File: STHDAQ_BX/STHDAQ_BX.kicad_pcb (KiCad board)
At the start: 2 copper layers, 36 x 56 mm, 52 parts, among them J1 532611071, P1 S2B-PH-SM4-TB, U1 ADS1256IDBR, U2 ADP151AUJZ-3.0-R7, U3 OPA350UA, U4 REF5025AIDR, U5 102010448, U6 LT1461AIS8-5-PBF, Y1 ABLS-8MHZ-K4T

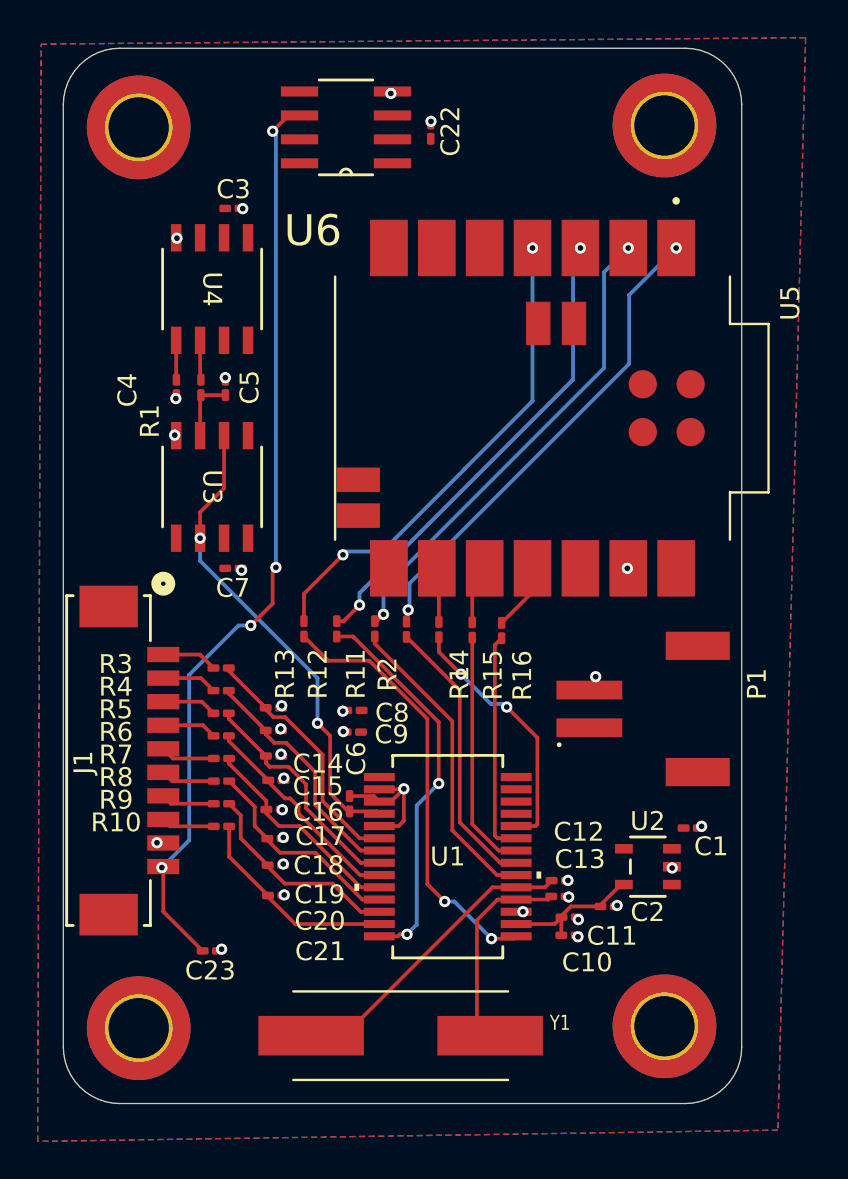
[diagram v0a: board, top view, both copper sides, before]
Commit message: Changes in BX
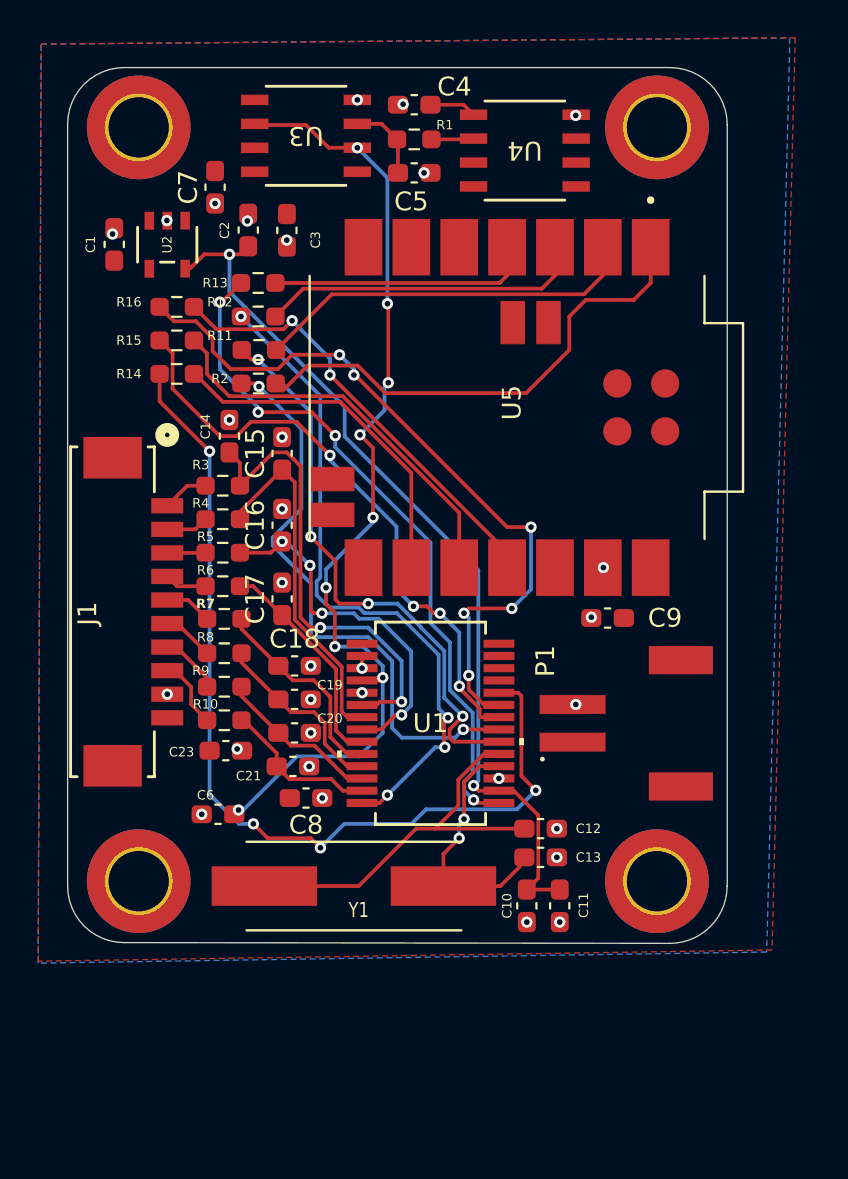
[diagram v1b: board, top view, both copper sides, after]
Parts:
- removed C22: 1u, Capacitor_SMD:C_0201_0603Metric_Pad0.64x0.40mm_HandSolder
- removed U6: LT1461AIS8-5-PBF, daFootprintsBX:SOIC127P600X175-8N
- C1, C10, C11, C12, C13, C14, C15, C16, C17, C18, C19, C2, C20, C21, C23, C3, C4, C5, C6, C7, C8, C9: footprint Capacitor_SMD:C_0201_0603Metric_Pad0.64x0.40mm_HandSolder -> Capacitor_SMD:C_0603_1608Metric_Pad1.08x0.95mm_HandSolder
- R1, R10, R11, R12, R13, R14, R15, R16, R2, R3, R4, R5, R6, R7, R8, R9: footprint Resistor_SMD:R_0201_0603Metric_Pad0.64x0.40mm_HandSolder -> Resistor_SMD:R_0603_1608Metric_Pad0.98x0.95mm_HandSolder
- moved C1 43.6 mm to (172.7, 90.4), turned to -90 degrees
- moved U2 41.7 mm to (175.5, 90.4), turned to -90 degrees
- moved C2 40.7 mm to (179.8, 89.6), turned to -90 degrees
- moved R16 24.3 mm to (176.0, 93.7), turned to 180 degrees
- moved R15 22.0 mm to (176.0, 95.5), turned to 180 degrees
- moved C7 20.2 mm to (178.1, 87.4), turned to 90 degrees
- moved C4 19.6 mm to (188.6, 83.0), turned to 0 degrees
- moved R14 19.4 mm to (176.0, 97.3), turned to 180 degrees
- moved U3 19.3 mm to (182.9, 84.6), turned to 180 degrees
- moved R13 18.5 mm to (180.3, 92.5), turned to 0 degrees
- moved U4 18.2 mm to (194.5, 85.4), turned to 180 degrees
- moved R1 17.4 mm to (188.6, 84.8), turned to 180 degrees
- moved R12 17.1 mm to (180.3, 94.2), turned to 0 degrees
- moved R11 16.0 mm to (180.4, 96.0), turned to 0 degrees
- moved R2 15.2 mm to (180.4, 97.8), turned to 0 degrees
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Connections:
- C1 pad 2: 5VCC -> 5BVCC
- C3 pad 2: 5VCC -> 5BVCC
- C7 pad 2: 5VCC -> 5BVCC
- C8 pad 2: 5VCC -> 5BVCC
- C9 pad 2: 5VCC -> 5BVCC
- P1 pad 1: 5VCC -> 5BVCC
- U1 pad 1: 5VCC -> 5BVCC
- U2 pad 1: 5VCC -> 5BVCC
- U2 pad 3: 5VCC -> 5BVCC
- U3 pad 7: 5VCC -> 5BVCC
- U4 pad 2: 5VCC -> 5BVCC
- U5 pad VUSB: 5VCC -> 5BVCC
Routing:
- net 5BVCC: track 49.1 -> 0.00 mm, vias 4 -> 0
- net REF3.3: track 7.63 -> 47.4 mm, vias 0 -> 2
- net /SCLK: track 13.6 -> 49.7 mm, vias 2 -> 4
- net /DIN: track 11.8 -> 39.2 mm, vias 0 -> 6
- net REF2.5: track 25.5 -> 52.9 mm, vias 2 -> 9
- net Net-(U5-D10/MOSI): track 3.57 -> 23.7 mm, vias 0 -> 2
- net /DOUT: track 12.8 -> 32.1 mm, vias 0 -> 4
- net Net-(U5-D9/MISO): track 3.14 -> 21.4 mm
- net /DRDY: track 14.9 -> 31.2 mm, vias 0 -> 2
- net Net-(U5-D8/SCK): track 2.89 -> 18.7 mm
- net /SYNC/PDWN: track 20.8 -> 35.2 mm, vias 2 -> 4
- net /CS: track 16.4 -> 30.4 mm, vias 0 -> 4
- net /RESET: track 23.1 -> 37.0 mm, vias 2 -> 4
- net Net-(U5-A3/D3): track 27.0 -> 14.0 mm, vias 2 -> 0
- net /S1+: track 13.3 -> 24.9 mm, vias 0 -> 2
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- added copper zone on F.Cu, net 5BVCC
- removed copper zone on F.Cu, net 5VCC
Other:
- board size 36 x 56 mm -> 35 x 46.5 mm
